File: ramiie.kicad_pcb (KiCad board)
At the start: 4 copper layers, 99.9 x 61.1 mm, 65 parts, among them J1 Memory Expansion, U1 EPM7128S, U2 4M x 4, U3 4M x 4, U4 4M x 4, U5 4M x 4, U6 ROM, U7 LD1117S33, U8 W25Q128, U9 W25Q128

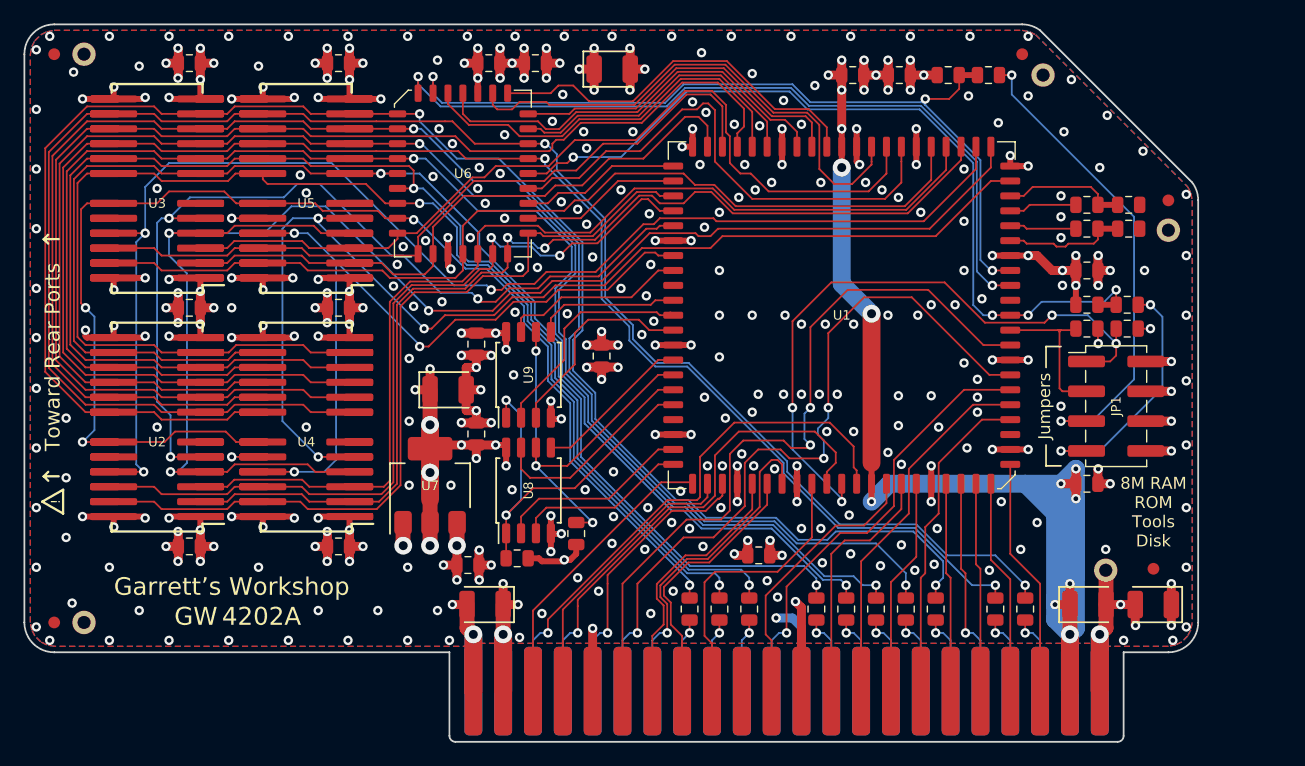
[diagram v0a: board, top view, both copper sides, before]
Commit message: did a lot
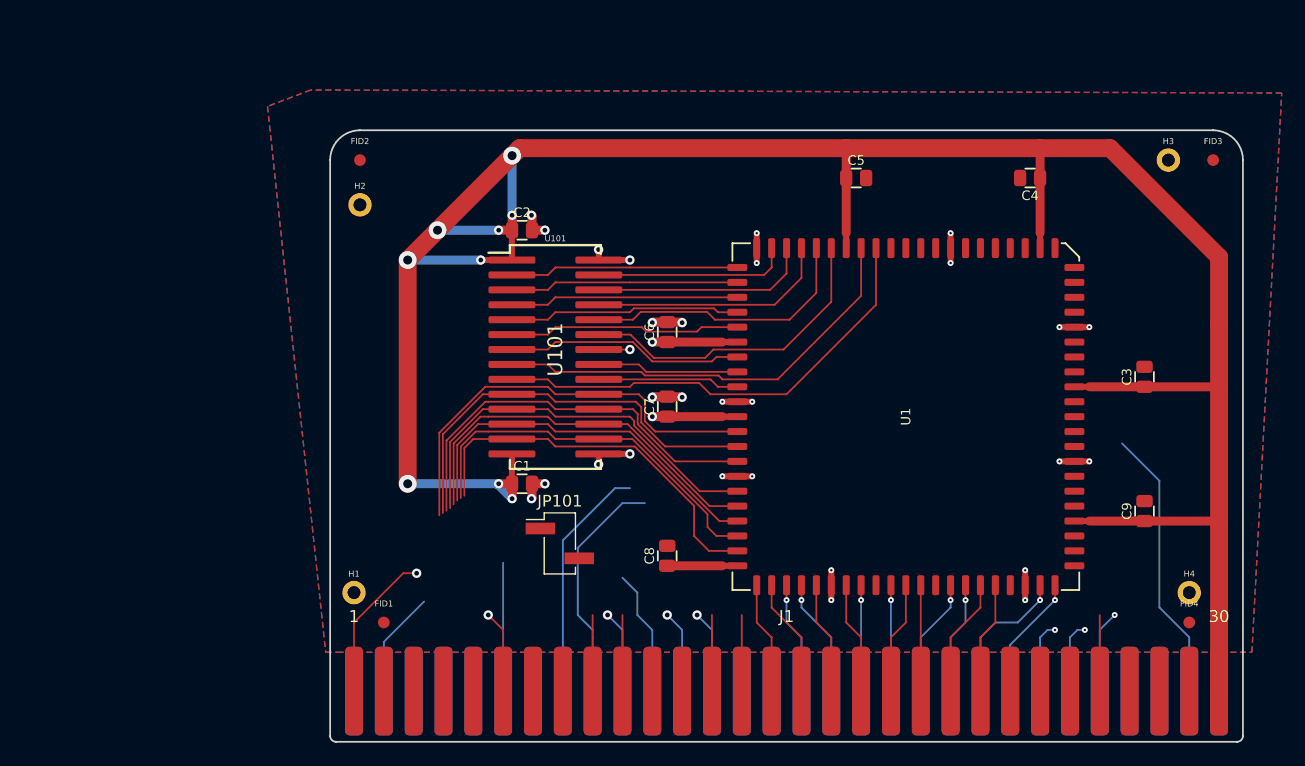
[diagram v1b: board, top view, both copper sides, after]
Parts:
- removed C10, C11, C12, C13, C14, C15, C16, C17, C18, C19: 100n, Capacitor_SMD:C_0805_2012Metric
- removed C20, C21, C22, C23, C24: 33u, stdpads:CP_EIA-3528
- removed FD1, FD2, FD3, FD4, FD5: Fiducial, stdpads:Fiducial
- removed H5: , stdpads:PasteHole_1.1mm_PTH
- removed JP1: Jumpers, stdpads:SMDHeader_2x04_P2.54mm_Vertical
- removed R1, R2, R5, R6: 820, Resistor_SMD:R_0805_2012Metric
- removed R10, R11, R12, R13, R14, R15, R16, R7, R8, R9: 100, Resistor_SMD:R_0805_2012Metric
- removed R17, R18, R19, R20, R3, R4: 10k, Resistor_SMD:R_0805_2012Metric
- removed U2, U3, U4, U5: 4M x 4, stdpads:SOP-24-26-300mil
- removed U6: ROM, stdpads:PLCC-32
- removed U7: LD1117S33, stdpads:SOT-223
- removed U8, U9: W25Q128, stdpads:SOIC-8_5.3mm
- added FID1: Fiducial, stdpads:Fiducial, F.Cu at (50.8, 129.5)
- added FID2: Fiducial, stdpads:Fiducial, F.Cu at (48.8, 90.2)
- added FID3: Fiducial, stdpads:Fiducial, F.Cu at (121.4, 90.2)
- added FID4: Fiducial, stdpads:Fiducial, F.Cu at (119.4, 129.5)
- added JP101: Jumper_NO_Small, Connector_PinHeader_2.54mm:PinHeader_1x02_P2.54mm_Vertical_SMD_Pin1Left, F.Cu at (65.8, 122.8)
- added U101: 2M x 8, stdpads:SOJ-28-300mil, F.Cu at (65.4, 106.9)
- C1, C2: value 10p -> 100n; footprint Capacitor_SMD:C_0805_2012Metric -> stdpads:C_0805
- C3, C4, C5, C6, C7, C8, C9: footprint Capacitor_SMD:C_0805_2012Metric -> stdpads:C_0805
- J1: value Memory Expansion -> AppleIIeAux; footprint stdpads:Apple_IIGS-MemoryExpansion -> stdpads:AppleIIeAux_Edge
- U1: value EPM7128S -> EPM7128SL84
- moved C9 89.8 mm to (115.6, 120.1), turned to 90 degrees
- moved H2 59.2 mm to (48.8, 94.0)
- moved C1 56.8 mm to (62.6, 117.7)
- moved C2 51.6 mm to (62.6, 96.1)
- moved H1 51.3 mm to (48.3, 127.0)
- moved C8 45.8 mm to (74.9, 123.9), turned to 90 degrees
- moved C7 42.4 mm to (74.9, 111.2), turned to 90 degrees
- moved C5 32.8 mm to (91.0, 91.7)
- moved C6 26.1 mm to (74.9, 104.8), turned to 90 degrees
- moved C4 17.5 mm to (105.8, 91.7), turned to 180 degrees
- moved C3 10.3 mm to (115.6, 108.6), turned to 90 degrees
- moved U1 10.2 mm to (95.2, 112.0), turned to 270 degrees
- moved H4 7.36 mm to (119.4, 127.0)
- moved H3 5.97 mm to (117.6, 90.2)
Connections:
- C1 pad 1: /CRASd -> +5V
- C2 pad 1: Net-(C2-Pad1) -> +5V
- J1 pad 1: GND -> /3.58M
- J1 pad 10: /FRA7 -> /RA1
- J1 pad 11: +5V -> /ROMEN1
- J1 pad 12: /~FWE~ -> /ROMEN2
- J1 pad 13: /FRA0 -> /RA4
- J1 pad 14: /FRA2 -> /RA5
- J1 pad 15: /FRA1 -> /V7
- J1 pad 16: /FD7 -> /MD7
- J1 pad 17: /~CCAS~ -> /MD6
- J1 pad 18: /CROW0 -> /V6
- J1 pad 19: /CROW1 -> /V5
- J1 pad 2: +5V -> /Vid7M
- J1 pad 20: /~CROMSEL~ -> /MD5
- J1 pad 21: +5V -> /MD4
- J1 pad 22: GND -> /V4
- J1 pad 23: GND -> /PHI0
- J1 pad 24: +5V -> /~CLRGAT~
- J1 pad 25: /FD0 -> /~80VID~
- J1 pad 26: /~CSEL~ -> /~EN80~
- J1 pad 27: GND -> /~ALTVID~
- J1 pad 28: /FD6 -> /~SEROUT~
- J1 pad 29: /FD4 -> /~ENVID~
- J1 pad 3: /FRA9 -> /~SYNC~
- J1 pad 30: /FD5 -> +5V
- J1 pad 31: /PH2 -> GND
- J1 pad 32: /ABORT -> /14M
- J1 pad 33: /FD3 -> /~PCAS~
- J1 pad 34: GND -> /~LDPS~
- J1 pad 35: /~CRAS~ -> /R~W~80
- J1 pad 36: /FD1 -> /PHI1
- J1 pad 37: /FA10 -> /~CASEN~
- J1 pad 38: /FA11 -> /V3
- J1 pad 39: /FA12 -> /MD3
- J1 pad 4: /FRA8 -> /~PRAS~
- J1 pad 40: /FA13 -> /MD2
- J1 pad 41: /FA14 -> /V2
- J1 pad 42: /FA15 -> /V1
- J1 pad 43: +5V -> /MD1
- J1 pad 44: GND -> /MD0
- J1 pad 5: /FD2 -> /VC
- J1 pad 6: /FRA6 -> /~C07X~
- J1 pad 7: /FRA3 -> /~WNDW~
- J1 pad 8: /FRA4 -> /SEGA
- J1 pad 9: /FRA5 -> /RA7
- U1 pad 1: /~8MEG~ -> /PHI1
- U1 pad 10: /FA13 -> /7M
- U1 pad 11: /FA14 -> /3.58M
- U1 pad 12: /FA15 -> Net-(U1-Pad12)
- U1 pad 13: +3V3 -> +5V
- U1 pad 15: /FA11 -> Net-(U1-Pad15)
- U1 pad 16: /FD1 -> Net-(U1-Pad16)
- U1 pad 17: /~FWE~ -> Net-(U1-Pad17)
- U1 pad 18: /~CCAS~ -> Net-(U1-Pad18)
- U1 pad 2: /~CROMSEL~ -> /Q3
- U1 pad 20: /FD6 -> Net-(U1-Pad20)
- U1 pad 21: /~ROMEN~ -> Net-(U1-Pad21)
- U1 pad 22: /ROMA11 -> Net-(U1-Pad22)
- U1 pad 24: /ROMA12 -> /RA10
- U1 pad 25: /ROMA15 -> /RA11
- U1 pad 26: +3V3 -> +5V
- U1 pad 27: Net-(C2-Pad1) -> /~CAS~
- U1 pad 28: Net-(R2-Pad2) -> /RD4
- U1 pad 29: /CRAS -> /RD5
- U1 pad 30: /CRASd -> /RD6
- U1 pad 31: /~RAS~1 -> /RD7
- U1 pad 33: /~WE~ -> /RD0
- U1 pad 34: /~CAS~0 -> /RD1
- U1 pad 35: /D0 -> /RD2
- U1 pad 36: /D1 -> /RD3
- U1 pad 37: /D7 -> /R~WE~
- U1 pad 38: +3V3 -> +5V
- U1 pad 39: /ROM~OE~ -> /~RAS~
- U1 pad 4: /FD3 -> Net-(U1-Pad4)
- U1 pad 40: /D5 -> /RA9
- U1 pad 41: /ROMR~W~ -> /RA8
- U1 pad 44: /ROMA17 -> /RA7
- U1 pad 45: /ROMA14 -> /RA0
- U1 pad 46: /ROMA18 -> /RA6
- U1 pad 48: /ROMA13 -> /RA1
- U1 pad 49: /ROMA16 -> /RA5
- U1 pad 5: /~CRAS~ -> /~CASEN~
- U1 pad 50: /A5 -> /RA2
- U1 pad 51: /D6 -> /RA4
- U1 pad 52: /D4 -> /RA3
- U1 pad 53: +3V3 -> +5V
- U1 pad 54: /ROMA10 -> /V7
- U1 pad 55: /ROM~CS~ -> /MD7
- U1 pad 56: /D3 -> /V0
- U1 pad 57: /D2 -> /MD0
- U1 pad 58: /~RAS~0 -> /MD6
- U1 pad 6: /FA10 -> /AN3
- U1 pad 60: /~CAS~1 -> /V6
- U1 pad 61: /F1D3 -> /MD1
- U1 pad 63: /F1D0 -> /V1
- U1 pad 64: /F1D1 -> /V5
- U1 pad 65: /F1D2 -> /MD5
- U1 pad 66: +3V3 -> +5V
- U1 pad 67: /F0D0 -> /V2
- U1 pad 68: /Fclk -> /MD2
- U1 pad 69: /F0D3 -> /MD4
- U1 pad 70: /F~CS~ -> /V4
- U1 pad 73: /F0D1 -> /MD3
- U1 pad 74: /F0D2 -> /V3
- U1 pad 75: /FD0 -> Net-(U1-Pad75)
- U1 pad 76: /~CSEL~ -> /PHI0
- U1 pad 77: /CROW0 -> Net-(U1-Pad77)
- U1 pad 78: +3V3 -> +5V
- U1 pad 79: /FD4 -> /~EN80~
- U1 pad 8: /FA12 -> /R~W~
- U1 pad 80: /FD5 -> Net-(U1-Pad80)
- U1 pad 81: /FD7 -> /14M
- U1 pad 83: /PH2 -> /14M
- U1 pad 84: /CROW1 -> /R~W~80
- U1 pad 9: /FD2 -> /~C07X~
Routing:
- net GND: track 214.2 -> 40.0 mm, vias 331 -> 29
- net /A4: track 154.7 -> 0.00 mm, vias 2 -> 0
- net /A3: track 147.2 -> 0.00 mm, vias 2 -> 0
- net /A6: track 144.5 -> 0.00 mm, vias 2 -> 0
- net /A2: track 138.7 -> 0.00 mm, vias 2 -> 0
- net /~WE~: track 135.3 -> 0.00 mm, vias 3 -> 0
- net /A1: track 132.4 -> 0.00 mm, vias 2 -> 0
- net /A0: track 126.3 -> 0.00 mm, vias 2 -> 0
- net /A7: track 124.1 -> 0.00 mm, vias 2 -> 0
- net /A10: track 118.7 -> 0.00 mm, vias 2 -> 0
- net /A8: track 116.0 -> 0.00 mm, vias 2 -> 0
- net /~CAS~0: track 112.5 -> 0.00 mm, vias 3 -> 0
- net /A5: track 111.9 -> 0.00 mm
- net /A9: track 109.9 -> 0.00 mm, vias 4 -> 0
- net /~RAS~1: track 97.7 -> 0.00 mm, vias 3 -> 0
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- removed copper zone on In2.Cu, net +3V3
- removed copper zone on In2.Cu, net +5V
- removed copper zone on In1.Cu, net GND
- removed copper zone on In2.Cu, net GND
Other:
- board size 99.9 x 61.1 mm -> 77.7 x 52.1 mm
- rule via_min_drill: 0.3 -> 0.2
- rule via_min_size: 0.4 -> 0.508
- board text removed: "!"
- board text removed: "4202A"
- board text removed: "8M RAM ROM Tools Disk"
- board text removed: "8M RAM, 32M Disk"
- board text removed: "GW"
- board text removed: "Garrett’s Workshop"
- board text removed: "JLCJLCJLC"
- board text removed: "Jumpers"
- board text removed: "Toward Rear Ports"
- board text removed: "ZK, GF"
- board text removed: "for Apple IIgs"
